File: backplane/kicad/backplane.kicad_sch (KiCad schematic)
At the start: 14 parts, among them J1 Conn_01x02_Pin

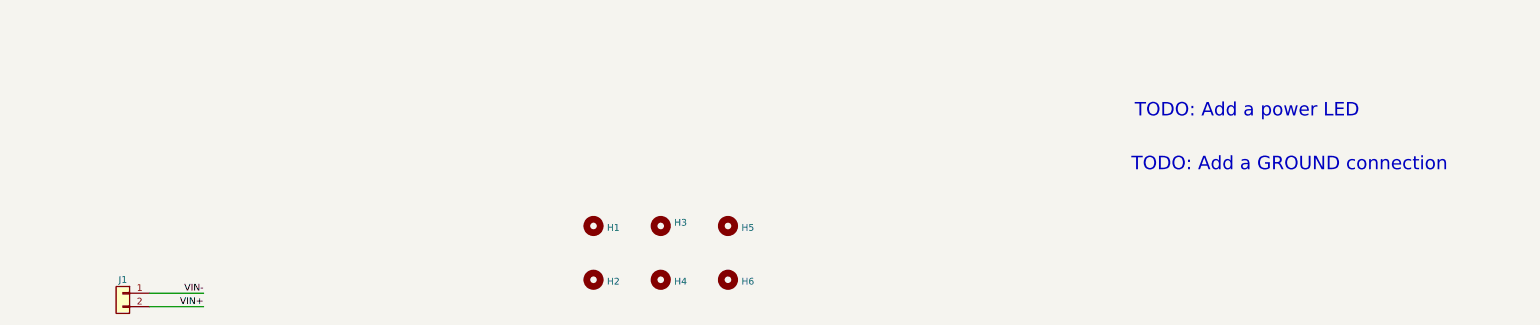
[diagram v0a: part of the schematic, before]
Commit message: Cleaned up TODOs for next version of backplane.
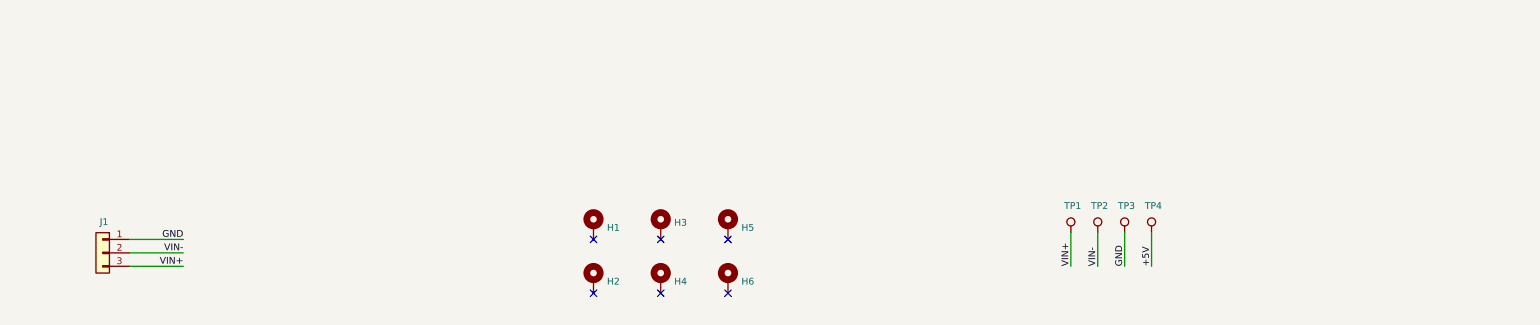
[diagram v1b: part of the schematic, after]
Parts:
- added TP1, TP2, TP3, TP4: TestPoint, common:Test_Pad, symbol Connector:TestPoint
- H1, H2, H3, H4, H5, H6: symbol Mechanical:MountingHole -> Mechanical:MountingHole_Pad
- J1: footprint backplane:JST_XH_B2B-XH-AM_1x02_P2.50mm_Vertical -> backplane:TerminalBlock_3P_7.62mm; symbol Connector_Generic:Conn_01x02 -> Connector_Generic:Conn_01x03; LCSC (none) -> C557662
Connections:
- net +5V: now also TP4.1
- net GND: now also J1.1 (Pin_1), TP3.1
- net VIN+: now also J1.3 (Pin_3), TP1.1; no longer J1.2 (Pin_2)
- net VIN-: now also J1.2 (Pin_2), TP2.1; no longer J1.1 (Pin_1)
- no-connect marks 0 -> 6
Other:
- note removed: "TODO: Add a GROUND connection"
- note removed: "TODO: Add a power LED"
